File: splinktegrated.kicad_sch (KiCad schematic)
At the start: 51 parts, among them J1 USB_C_Receptacle_USB2.0, J10 Ribbon, J11 Serial, J12 Conn_01x04_Female, J13 Conn_01x02_Female, J2 Conn_01x04_Female, J3 Conn_01x04_Female, J4 Conn_01x04_Female, J5 Conn_01x02, J6 Serial, J7 trackball, J8 Ribbon, J9 RGB, SW1 SW_SPST, SW2 SW_SPST, U1 RP2040, U2 GD25Q80CEIGR, U3 XC6210B332MR-G, U4 USBLC6-2P6, Y1 Crystal_GND24

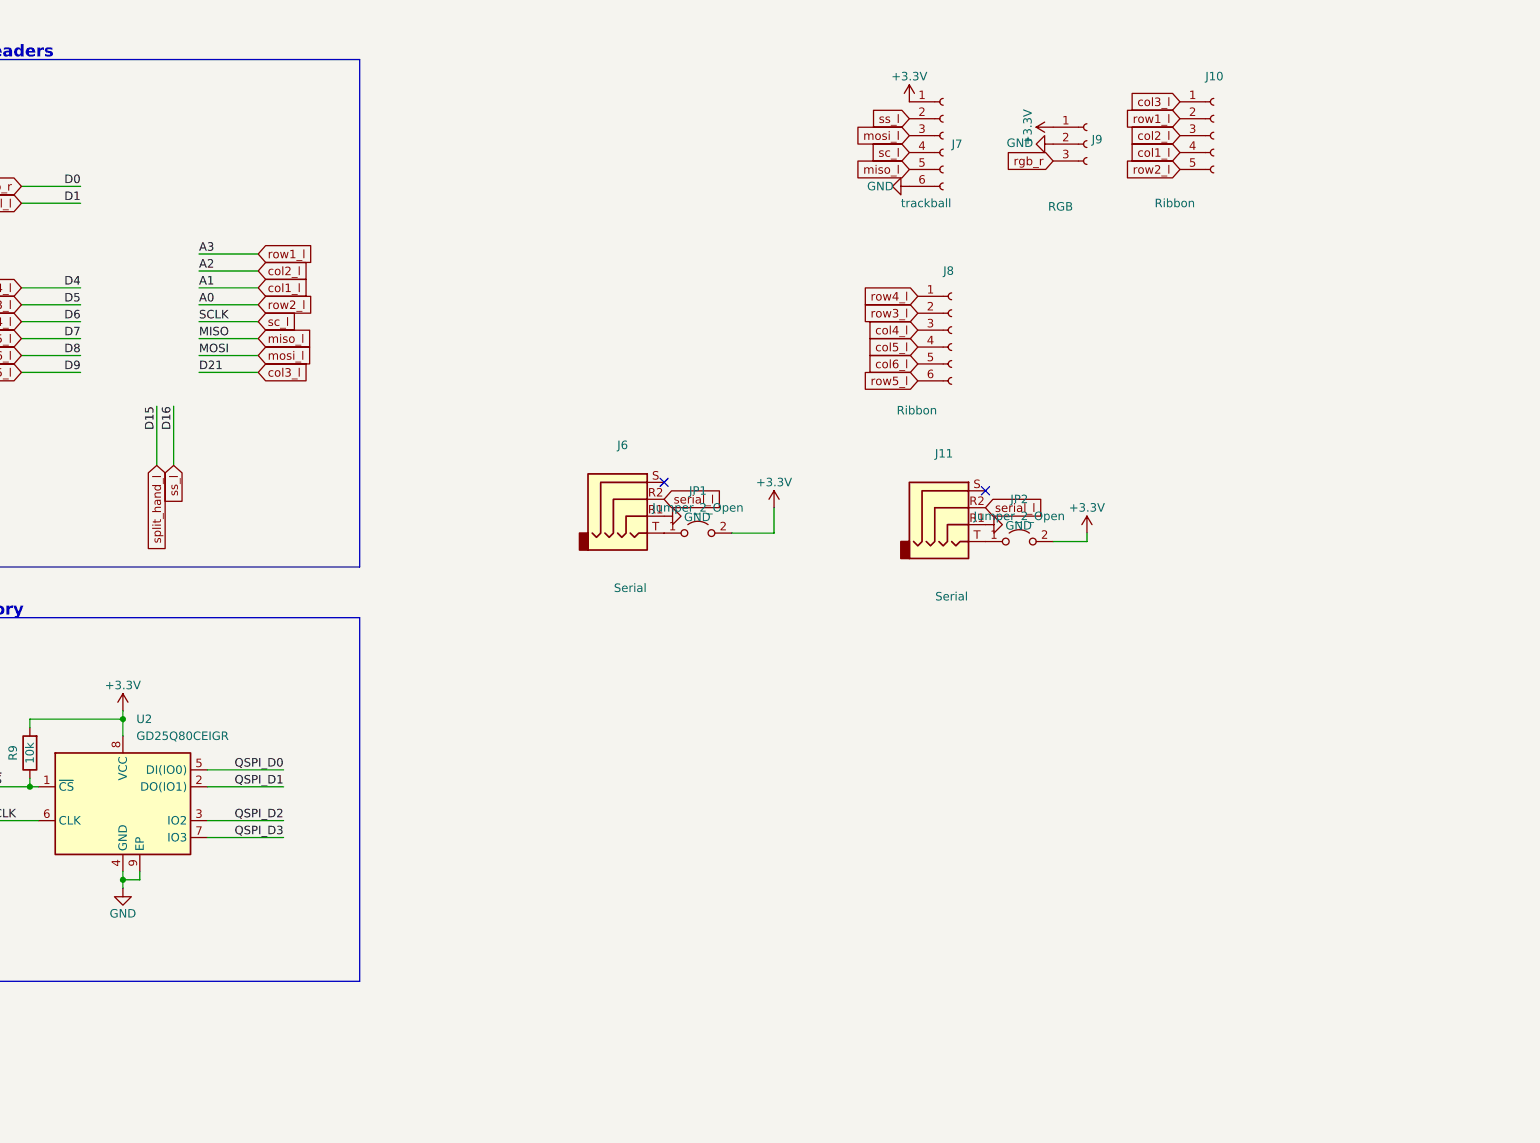
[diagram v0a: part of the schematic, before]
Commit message: memory, data line protection
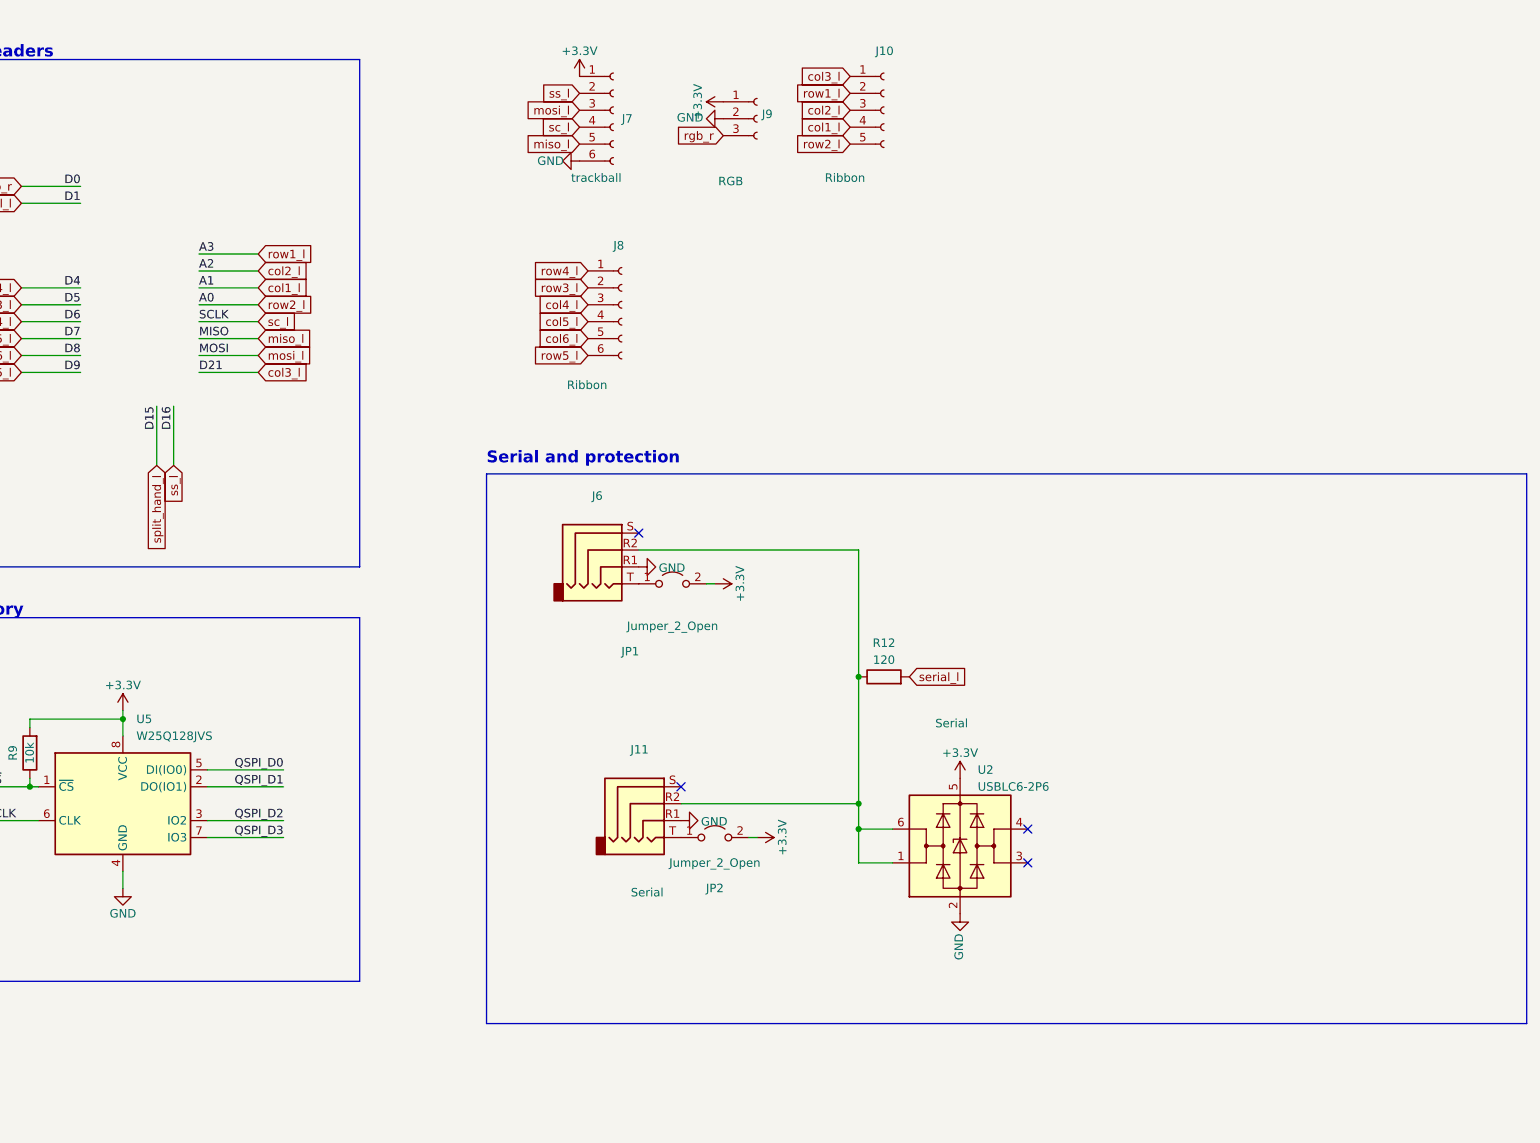
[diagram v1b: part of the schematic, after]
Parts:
- removed U2: GD25Q80CEIGR, 0xLib_Package_DFN_QFN:USON-8-1EP_3x2mm_P0.5mm_EP0.25x1.65mm, symbol Memory_Flash:W25Q32JVZP
- added R12: 120, Resistor_SMD:R_0402_1005Metric, symbol Device:R
- added U2: USBLC6-2P6, Package_TO_SOT_SMD:SOT-666, symbol Power_Protection:USBLC6-2P6
- added U5: W25Q128JVS, drawings:W25Q128JVPIQ, symbol Memory_Flash:W25Q128JVS
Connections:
- net +3V3: now also U2.5 (VBUS), U5.8 (VCC)
- net GND: now also U2.2 (GND), U5.4 (GND)
- net QSPI_D0: now also U5.5 (DI(IO0))
- net QSPI_D1: now also U5.2 (DO(IO1))
- net QSPI_D2: now also U5.3 (IO2)
- net QSPI_D3: now also U5.7 (IO3)
- net QSPI_SCLK: now also U5.6 (CLK)
- net QSPI_~{CS}: now also U5.1 (~{CS})
- net serial_l: now also R12.2; no longer J11.R2, J6.R2
- new net: J11.R2, J6.R2, R12.1, U2.1 (I/O1), U2.6 (I/O1)
- no-connect marks 16 -> 18
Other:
- note added: "Serial and protection"
- moved on the sheet: J10, J11, J6, J7, J8, J9, JP1, JP2
